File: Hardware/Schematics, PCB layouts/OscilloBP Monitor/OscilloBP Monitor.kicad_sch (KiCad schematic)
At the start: 8 parts, among them Q1 BSS138, U1 ZC323000, U2 MT3608

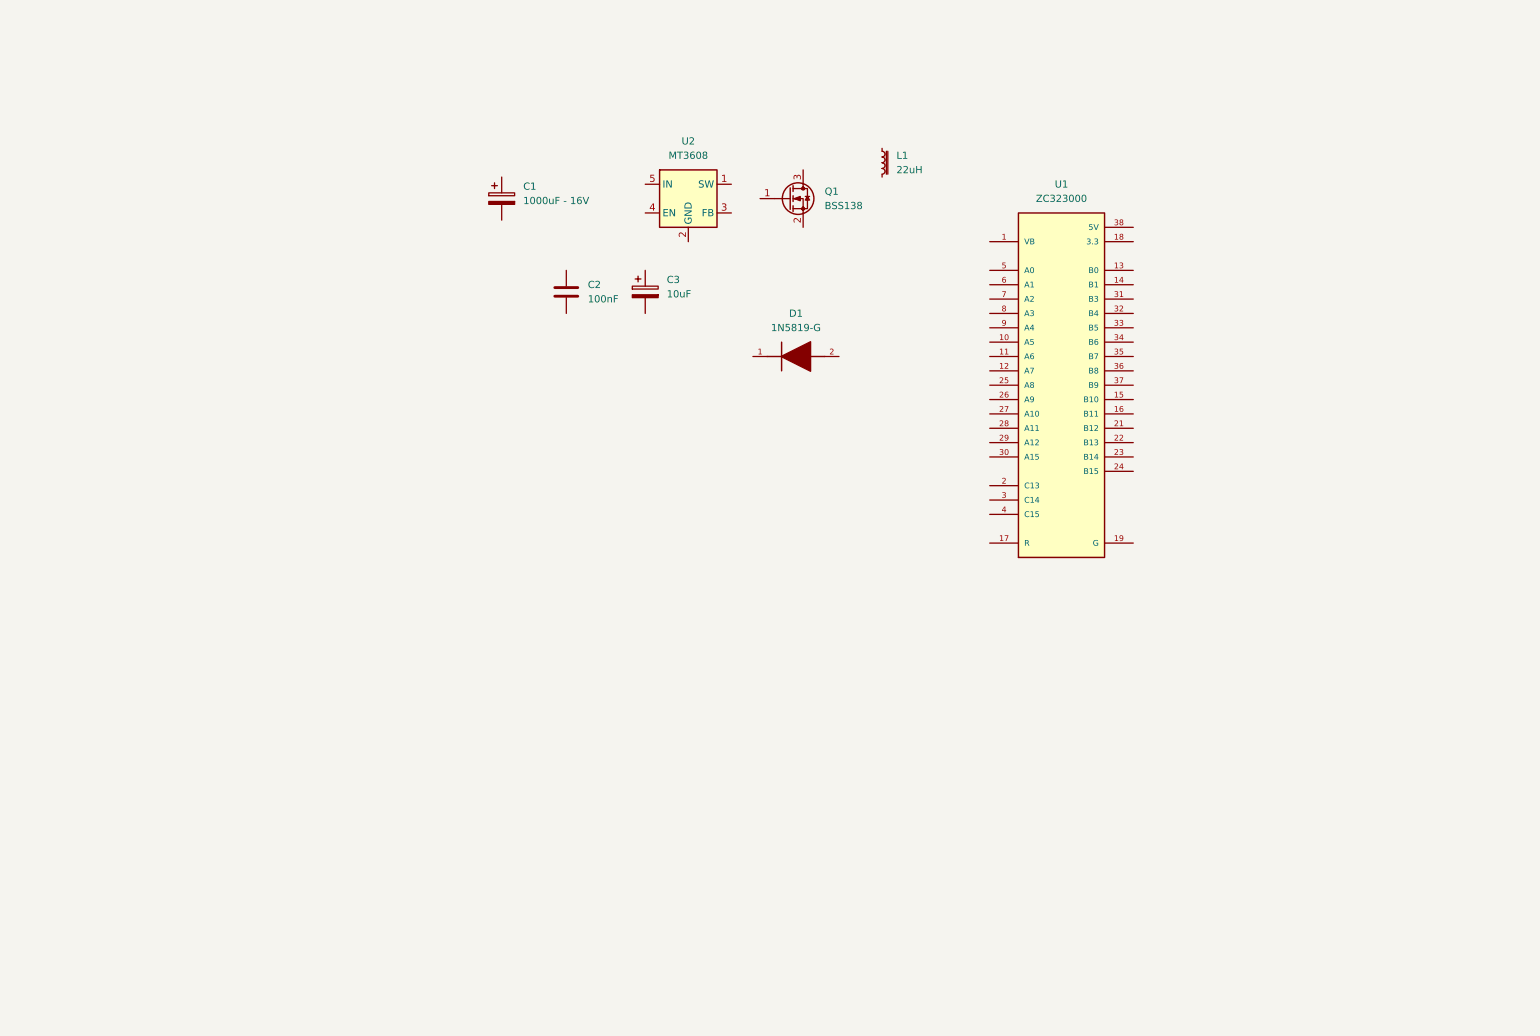
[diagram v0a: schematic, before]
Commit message: Thêm schematic.pdf
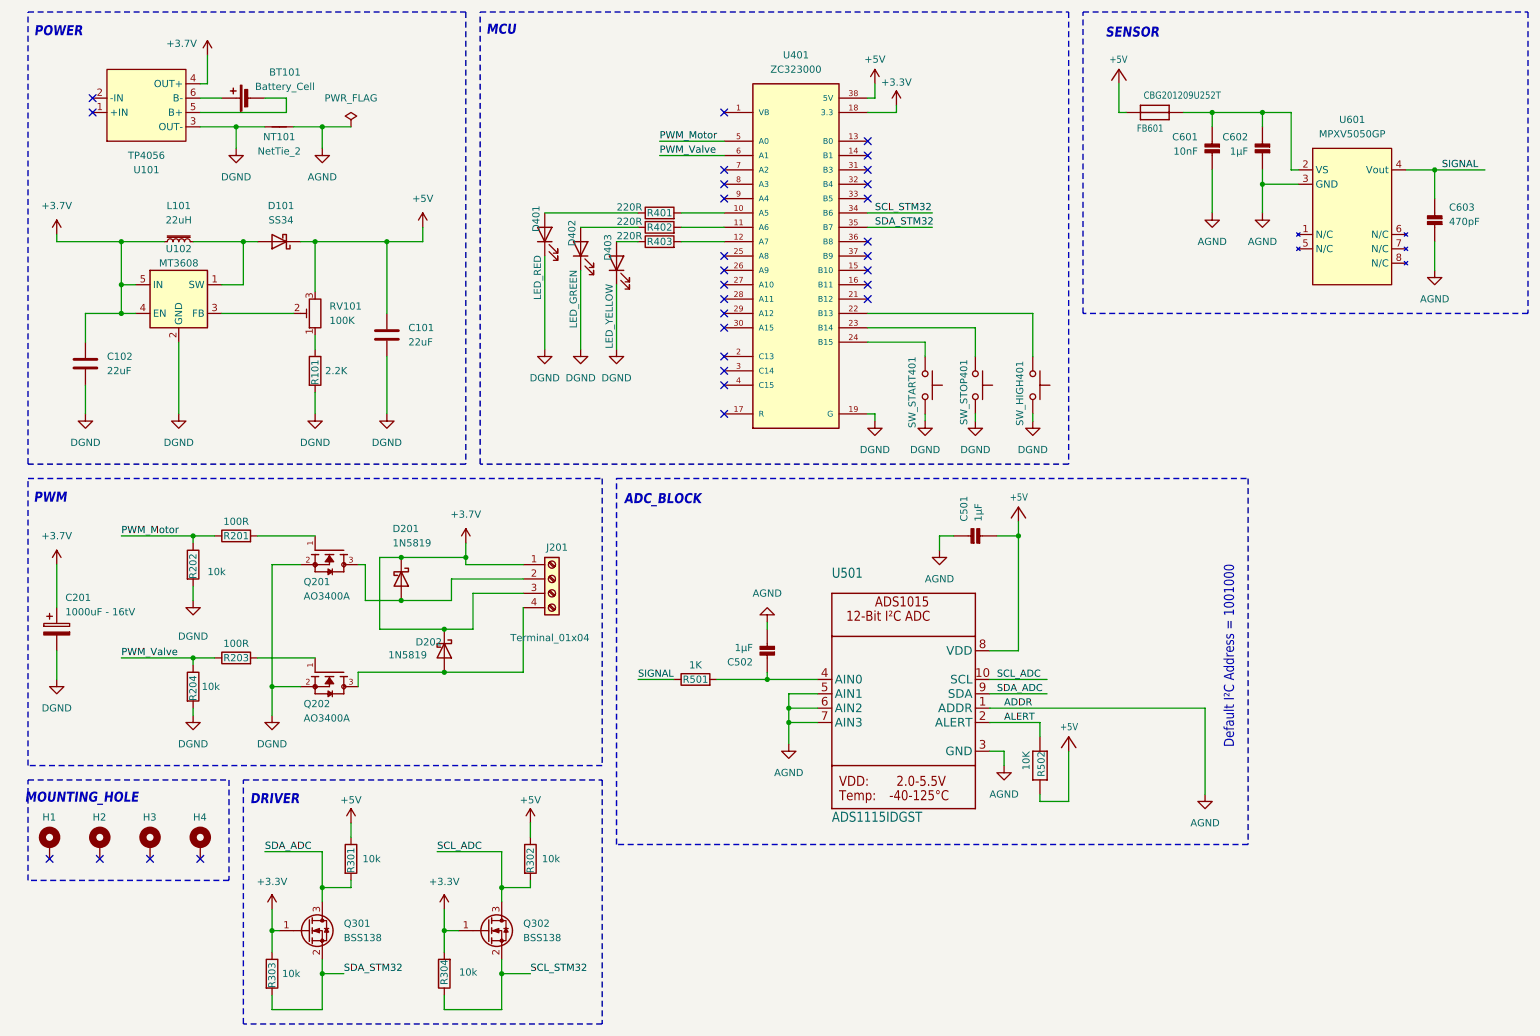
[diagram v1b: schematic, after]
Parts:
- removed C1: 1000uF - 16V, Capacitor_THT:CP_Radial_D16.0mm_P7.50mm, symbol Device:C_Polarized
- removed C2: 100nF, Capacitor_SMD:C_0603_1608Metric, symbol Device:C
- removed C3: 10uF, Capacitor_Tantalum_SMD:CP_EIA-1608-08_AVX-J_HandSolder, symbol Device:C_Polarized
- removed D1: 1N5819-G, 1N5819G:DIOAD1405W75L465D235, symbol 1N5819-G:1N5819-G
- added BT101: Battery_Cell, Battery1:1x18650, symbol Device:Battery_Cell
- added C101, C102: 22uF, Capacitor_SMD:C_1206_3216Metric_Pad1.33x1.80mm_HandSolder, symbol Device:C
- added C201: 1000uF - 16tV, Capacitor_THT:CP_Radial_D16.0mm_P7.50mm, symbol Device:C_Polarized
- added C501, C502, C602: 1µF, Capacitor_SMD:C_1206_3216Metric_Pad1.33x1.80mm_HandSolder, symbol Adafruit_ADS1115_16Bit_I2C_ADC-eagle-import:CAP_CERAMIC0805
- added C601: 10nF, Capacitor_SMD:C_1206_3216Metric_Pad1.33x1.80mm_HandSolder, symbol Adafruit_ADS1115_16Bit_I2C_ADC-eagle-import:CAP_CERAMIC0805
- added C603: 470pF, Capacitor_SMD:C_1206_3216Metric_Pad1.33x1.80mm_HandSolder, symbol Adafruit_ADS1115_16Bit_I2C_ADC-eagle-import:CAP_CERAMIC0805
- added D101: SS34, Diode_SMD:D_SMA, symbol Diode:SS34
- added D201, D202: 1N5819, Diode_THT:D_DO-41_SOD81_P10.16mm_Horizontal, symbol Diode:1N5819
- added D401: LED_RED, LED_THT:LED_D3.0mm, symbol Device:LED
- added D402: LED_GREEN, LED_THT:LED_D3.0mm, symbol Device:LED
- added D403: LED_YELLOW, LED_THT:LED_D3.0mm, symbol Device:LED
- added FB601: CBG201209U252T, Inductor_SMD:L_0805_2012Metric_Pad1.05x1.20mm_HandSolder, symbol Adafruit_ADS1115_16Bit_I2C_ADC-eagle-import:FERRITE0805
- added H1, H2, H3, H4: MountingHole_Pad, MountingHole_3.2mm_M3_Pad_Via_Silk:MountingHole_3.2mm_M3_Pad_Via_Silk, symbol Mechanical:MountingHole_Pad
- added J201: Terminal_01x04, TerminalBlock_KF:TerminalBlock_KF_1x04_P7.62mm_Vertical, symbol Connector:Screw_Terminal_01x04
- added NT101: NetTie_2, symbol Device:NetTie_2
- added Q201, Q202: AO3400A, AO3400A:SOT95P280X125-3N, symbol AO3400A:AO3400A
- added Q302: BSS138, Package_TO_SOT_SMD:SOT-23, symbol Transistor_FET:BSS138
- added R101: 2.2K, Resistor_SMD:R_1206_3216Metric_Pad1.30x1.75mm_HandSolder, symbol Device:R
- added R201, R203: 100R, Resistor_SMD:R_1206_3216Metric_Pad1.30x1.75mm_HandSolder, symbol Device:R
- added R202, R204, R301, R302, R303, R304: 10k, Resistor_SMD:R_1206_3216Metric_Pad1.30x1.75mm_HandSolder, symbol Device:R
- added R401, R402, R403: 220R, Resistor_SMD:R_1206_3216Metric_Pad1.30x1.75mm_HandSolder, symbol Device:R
- added R501: 1K, Resistor_SMD:R_1206_3216Metric_Pad1.30x1.75mm_HandSolder, symbol Device:R
- added R502: 10K, Resistor_SMD:R_1206_3216Metric_Pad1.30x1.75mm_HandSolder, symbol Adafruit_ADS1115_16Bit_I2C_ADC-eagle-import:RESISTOR0805
- added RV101: 100K, Potentiometer_THT:Potentiometer_Bourns_3296W_Vertical, symbol Device:R_Potentiometer_Trim
- added SW_HIGH401, SW_START401, SW_STOP401: SW_Push, Button_Switch_THT:SW_SPST_Omron_B3F-40xx, symbol Switch:SW_Push
- added U101: TP4056, TP4056_Module:TP4056_Module, symbol TP4056__Module:TP4056
- added U501: ADS1115IDGST, ADS1115:ADS1115_MSOP10, symbol Adafruit_ADS1115_16Bit_I2C_ADC-eagle-import:ADC_ADS1015
- added U601: MPXV5050GP, MPXV5050GP:SOIC127P600X175-8N, symbol MPXV5050GP:MPXV5050GP
- U401: renamed from U1; footprint STM32F103C8T6:STM32F103C8T6 -> ZC323000:MODULE_ZC323000
- renumbered L1 to L101, Q1 to Q301, U2 to U102
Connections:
- net 3.3 is gone; now on net +3.3V: U401.18 (3.3), U401.40 (3.3)
- net G is gone; now on net DGND: U401.19 (G), U401.20 (G), U401.39 (G)
- net +3.3V: now reaches Q301.1 (G)
- net +3.3V: now also Q302.1 (G), R303.1, R304.2
- net SDA_STM32: now reaches Q301.2 (S)
- net SDA_STM32: now also U401.35 (B7), R303.2
- net SDA_ADC: now reaches Q301.3 (D)
- net SDA_ADC: now also R301.2, U501.9 (SDA)
- net +3.7V: now reaches L101.1
- net +3.7V: now also U102.4 (EN), U102.5 (IN), C102.1, C201.1, D201.1 (K), D202.1 (K), J201.1 (Pin_1), J201.3 (Pin_3), U101.4 (OUT+)
- net at L101.2: now also U102.1 (SW), D101.2 (A)
- net at U401.10 (A5): now also R401.2
- net at U401.11 (A6): now also R402.2
- net at U401.12 (A7): now also R403.2
- net at U401.22 (B13): now also SW_HIGH401.1
- net at U401.23 (B14): now also SW_STOP401.1
- net at U401.24 (B15): now also SW_START401.1
- net SCL_STM32: now reaches U401.34 (B6)
- net SCL_STM32: now also Q302.2 (S), R304.1
- net +5V: now reaches U401.38 (5V)
- net +5V: now also C101.1, C501.2 (P$2), D101.1 (K), FB601.2 (P$2), R301.1, R302.1, R502.2, RV101.3, U501.8 (VDD)
- net PWM_Motor: now reaches U401.5 (A0)
- net PWM_Motor: now also R201.1, R202.1
- net PWM_Valve: now reaches U401.6 (A1)
- net PWM_Valve: now also R203.1, R204.1
- net DGND: now reaches U102.2 (GND)
- net DGND: now also C101.2, C102.2, C201.2, D401.1 (K), D402.1 (K), D403.1 (K), NT101.1, Q201.2, Q202.2, R101.2, R202.2, R204.2, SW_HIGH401.2, SW_START401.2, SW_STOP401.2, U101.3 (OUT-)
- net at U102.3 (FB): now also RV101.2
- new net: C502.1 (P$1), R501.2, U501.4 (AIN0)
- new net: D202.2 (A), J201.4 (Pin_4), Q202.3
- new net: Q201.1, R201.2
- new net: D401.2 (A), R401.1
- new net: C601.1 (P$1), C602.1 (P$1), FB601.1 (P$1), U601.2 (VS)
- new net: D201.2 (A), J201.2 (Pin_2), Q201.3
- new net: D403.2 (A), R403.1
- new net: Q202.1, R203.2
- new net: R101.1, RV101.1
- new net: BT101.2 (-), U101.5 (B+)
- new net: BT101.1 (+), U101.6 (B-)
- new net: D402.2 (A), R402.1
- new net AGND: C501.1 (P$1), C502.2 (P$2), C601.2 (P$2), C602.2 (P$2), C603.2 (P$2), NT101.2, U501.1 (ADDR), U501.3 (GND), U501.5 (AIN1), U501.6 (AIN2), U501.7 (AIN3), U601.3 (GND)
- new net ALERT: R502.1, U501.2 (ALERT)
- new net SCL_ADC: Q302.3 (D), R302.2, U501.10 (SCL)
- new net SIGNAL: C603.1 (P$1), R501.1, U601.4 (Vout)
- no-connect marks 0 -> 30
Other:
- note added: "ADC_BLOCK"
- note added: "DRIVER"
- note added: "Default I²C Address = 1001000"
- note added: "MCU"
- note added: "MOUNTING_HOLE"
- note added: "POWER"
- note added: "PWM"
- note added: "SENSOR"
- moved on the sheet: L101, Q301, U102, U401
